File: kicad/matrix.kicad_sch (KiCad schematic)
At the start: 175 parts, among them SW1 Esc, SW10 F9, SW11 F10, SW12 F11, SW13 F12, SW14 PrintScreen, SW15 ScrollLock, SW16 PauseBreak, SW17 Backspace, SW19 1, SW2 F1, SW20 2, SW21 3, SW22 4, SW23 5, SW24 6, SW25 7, SW26 8, SW27 9, SW28 0, SW29 -, SW3 F2, SW30 =, SW31 Backspace, SW32 Insert, SW33 Home, SW34 PgUp, SW35 Tab, SW36 Q, SW37 W, SW38 E, SW39 R, SW4 F3, SW40 T, SW41 Y, SW42 U, SW43 I, SW44 O, SW45 P, SW46 [, SW47 ], SW48 \, SW49 Delete, SW5 F4, SW50 End, SW51 PgDw, SW52 CapsLock, SW53 A, SW54 S, SW55 D, SW56 F, SW57 G, SW58 H, SW59 J, SW6 F5, SW60 K, SW61 L, SW62 ;, SW63 ', SW64 \ ISO, SW65 Enter, SW66 LShift, SW67 \ ISO, SW68 Z, SW69 X, SW7 F6, SW70 C, SW71 V, SW72 B, SW73 N, SW74 M, SW75 ,, SW76 ., SW77 /, SW78 RShift (???), SW79 RShift, SW8 F7, SW80 Up, SW81 LCtrl, SW82 LAlt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

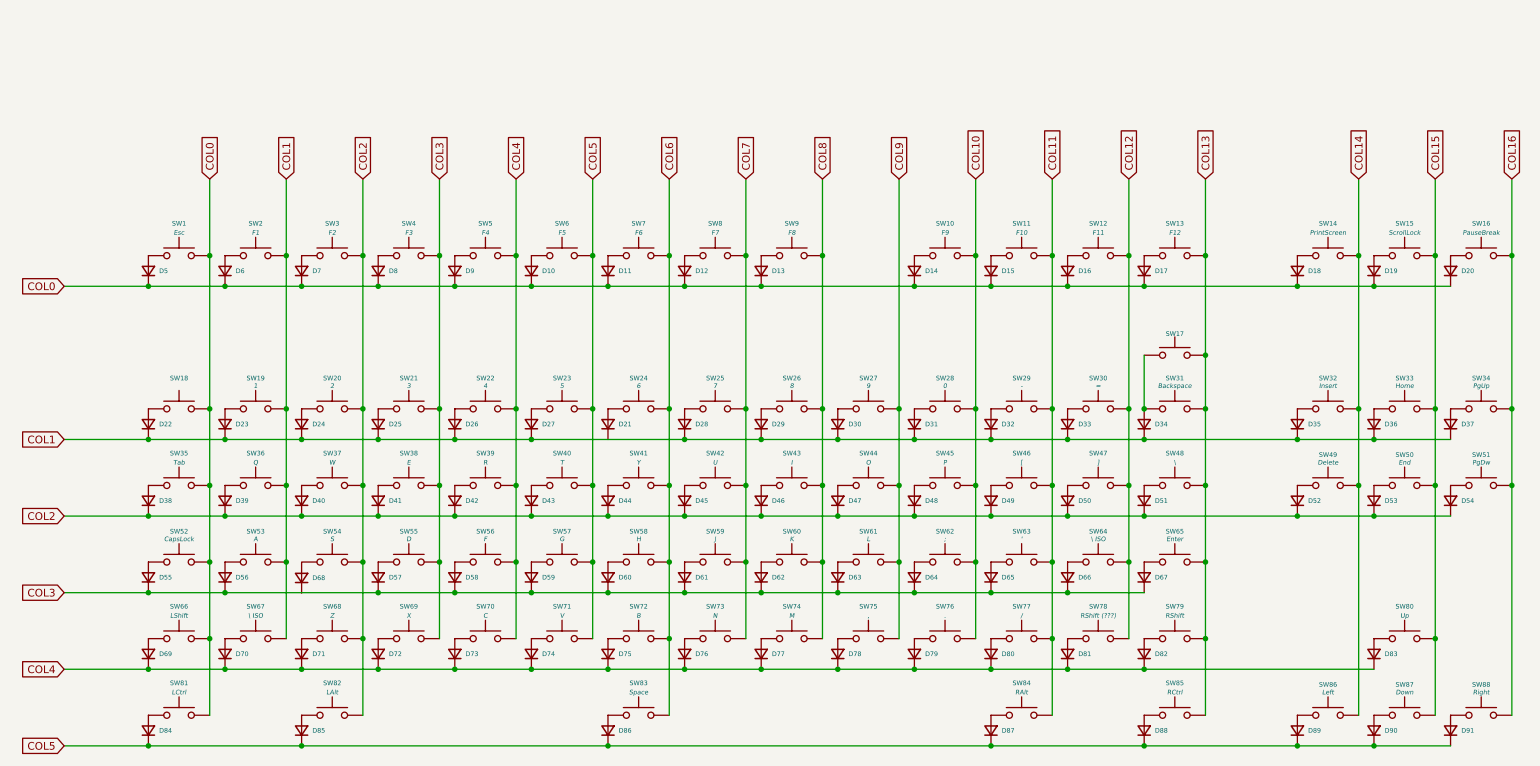
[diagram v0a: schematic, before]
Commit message: update
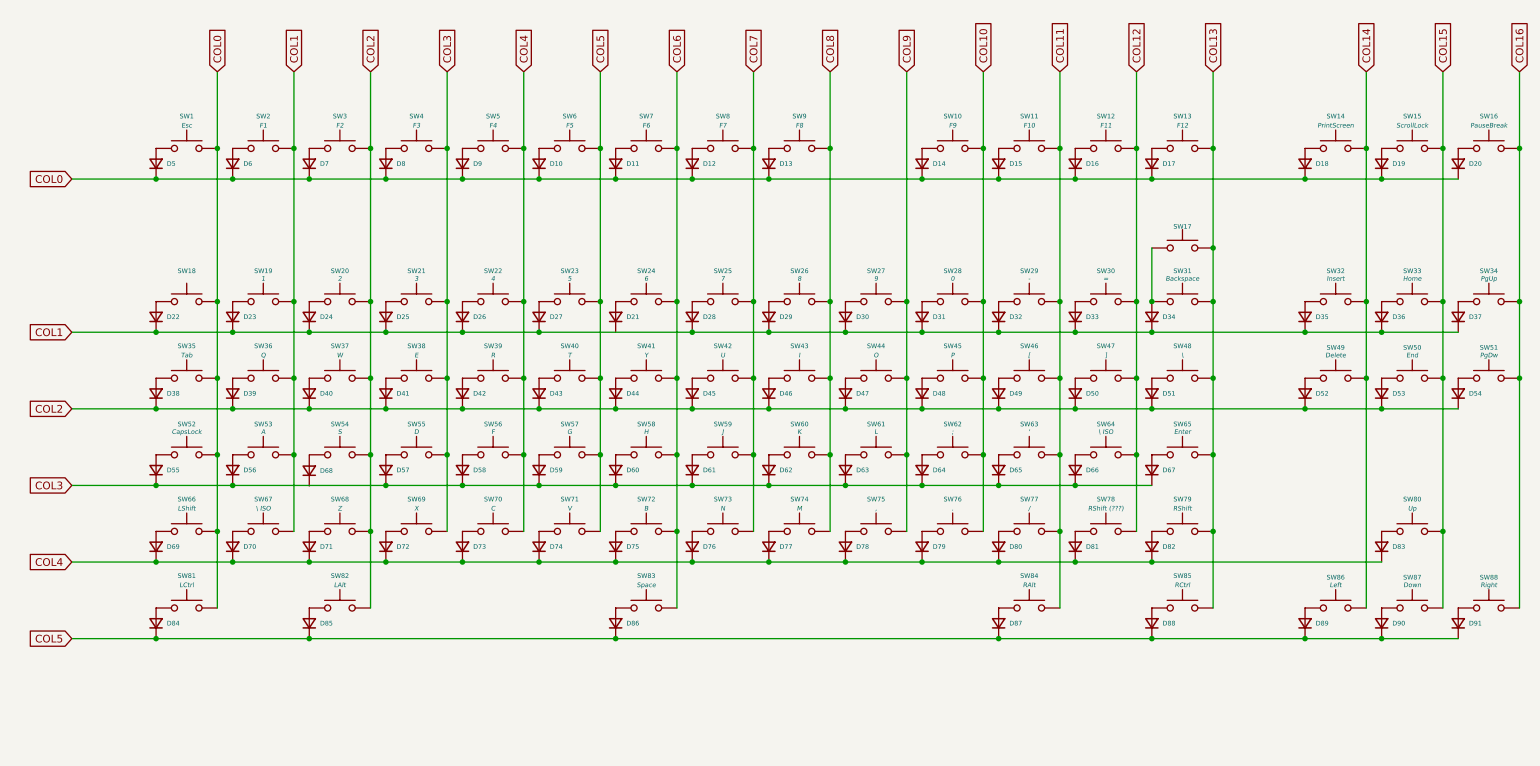
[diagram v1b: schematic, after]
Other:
- moved on the sheet: D10, D11, D12, D13, D14, D15, D16, D17, D18, D19, D20, D21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
